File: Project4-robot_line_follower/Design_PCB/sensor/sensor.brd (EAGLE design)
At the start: 134.9 x 70.1 mm, 57 parts

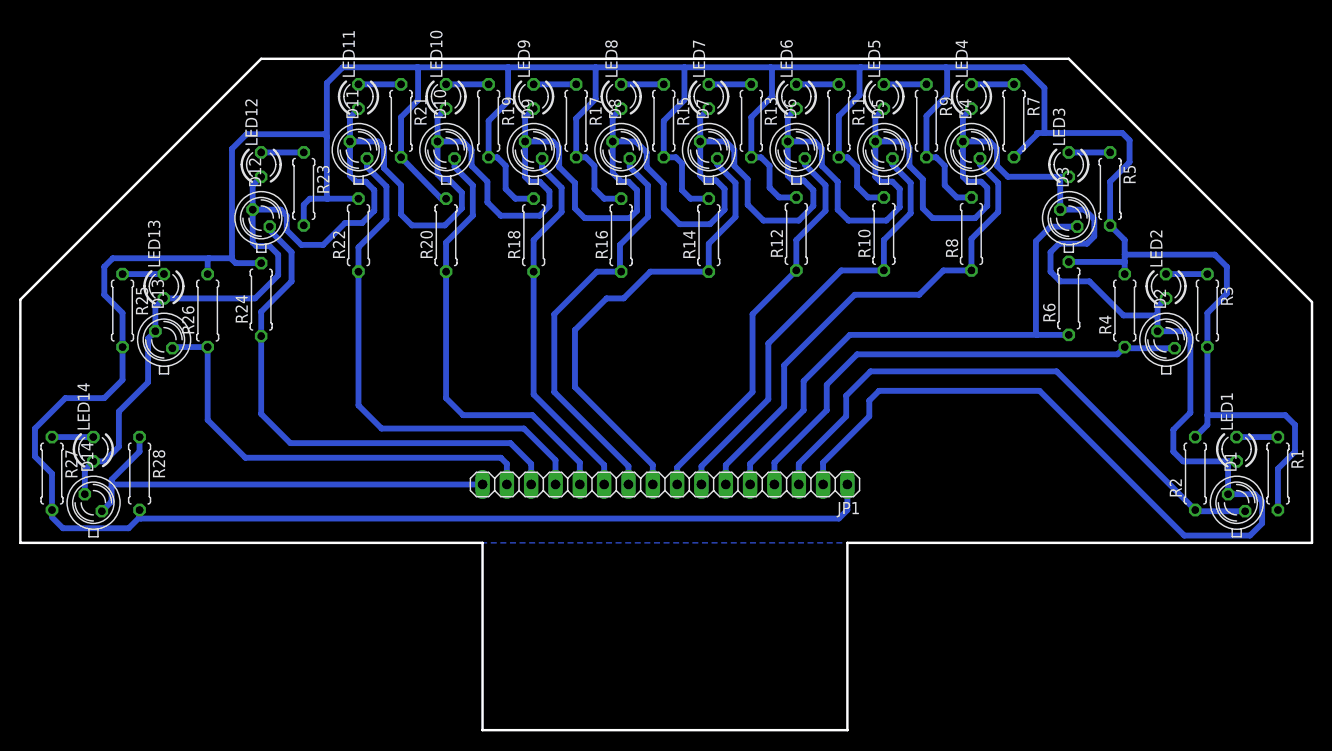
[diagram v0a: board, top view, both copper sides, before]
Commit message: rename file
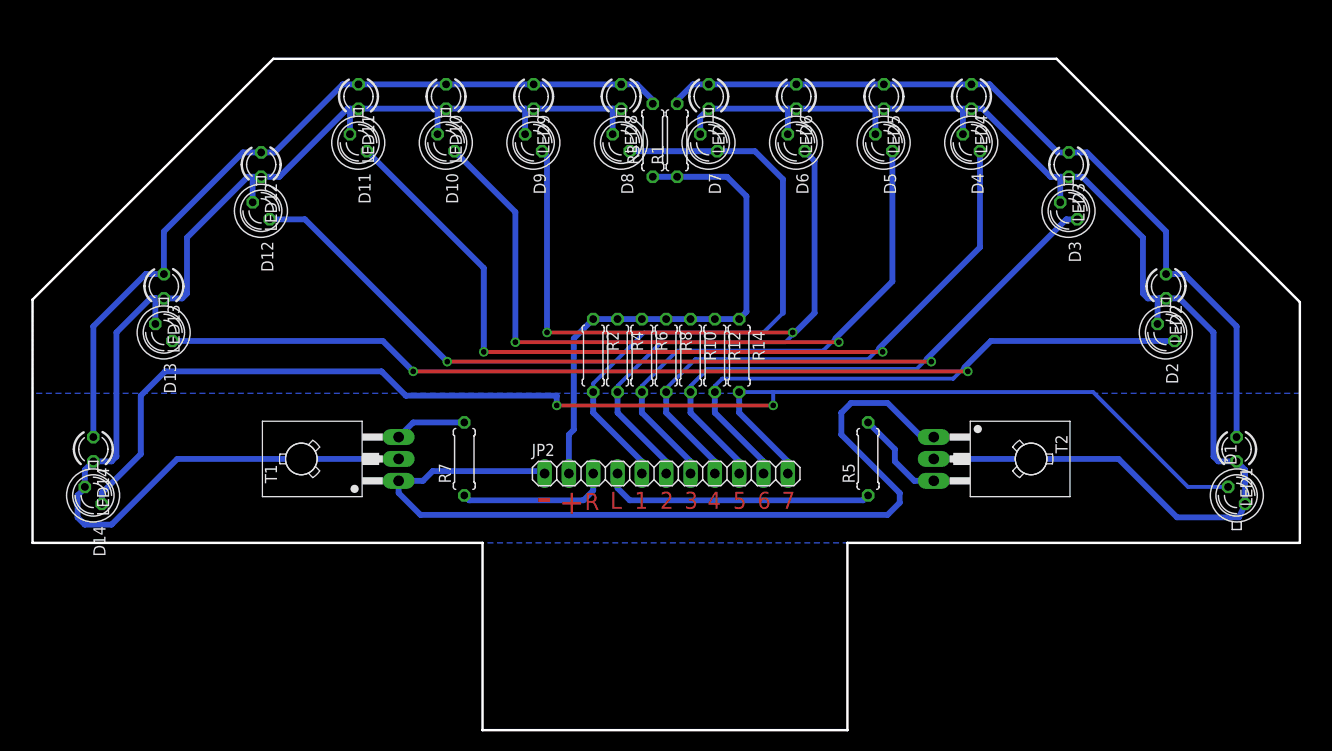
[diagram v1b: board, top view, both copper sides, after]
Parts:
- removed JP1: (no value), pinhead:1X16
- removed R11, R13, R15, R17, R19, R21, R23, R25, R27, R9: 470, rcl:0207/7
- removed R16, R18, R20, R22, R24, R26, R28: 22K, rcl:0207/7
- added JP2: (no value), pinhead:1X11
- added T1, T2: BD139, transistor:TO126
- R1, R3: value 470 -> 56
- R5, R7: value 470 -> 330
- moved R1 71.7 mm to (88.3, 72.1), turned to 90 degrees
- moved R7 67.4 mm to (66.0, 38.9), turned to 90 degrees
- moved R2 64.1 mm to (79.5, 49.7), turned to 270 degrees
- moved R3 60.6 mm to (85.7, 72.1), turned to 90 degrees
- moved R4 53.2 mm to (82.0, 49.7), turned to 270 degrees
- moved R6 45.0 mm to (84.6, 49.7), turned to 270 degrees
- moved R5 37.9 mm to (108.2, 38.9), turned to 90 degrees
- moved R8 34.3 mm to (87.1, 49.7), turned to 270 degrees
- moved R10 23.9 mm to (89.7, 49.7), turned to 270 degrees
- moved R12 15.3 mm to (92.2, 49.7), turned to 270 degrees
- moved R14 13.0 mm to (94.7, 49.7), turned to 270 degrees
- moved D1 0.76 mm to (146.7, 35.1)
- moved D10 0.76 mm to (64.1, 71.9), turned to 270 degrees
- moved D11 0.76 mm to (55.0, 71.9), turned to 270 degrees
- moved D12 0.76 mm to (44.8, 64.8), turned to 270 degrees
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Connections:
- removed net 10: D10.A, JP1.12, R20.1
- removed net 11: D11.A, JP1.13, R22.1
- removed net 12: D12.A, JP1.14, R24.1
- removed net 13: D13.A, JP1.15, R26.1
- removed net 14: D14.A, JP1.16, R28.1
- removed net 8: D8.A, JP1.10, R16.1
- removed net 9: D9.A, JP1.11, R18.1
- removed net N$11: LED6.K, R11.1
- removed net N$13: LED7.K, R13.1
- removed net N$15: LED8.K, R15.1
- removed net N$17: LED9.K, R17.1
- removed net N$19: LED10.K, R19.1
- removed net N$21: LED11.K, R21.1
- removed net N$23: LED12.K, R23.1
- removed net N$25: LED13.K, R25.1
- removed net N$27: LED14.K, R27.1
- removed net N$3: LED2.K, R3.1
- removed net N$5: LED3.K, R5.1
- removed net N$7: LED4.K, R7.1
- removed net N$9: LED5.K, R9.1
- new net D_KA: JP2.4, R5.1
- new net D_KI: JP2.3, R7.1
- new net LED_KA: LED1.A, LED2.A, LED3.A, LED4.A, LED5.A, LED6.A, LED7.A, R1.2
- new net LED_KI: LED10.A, LED11.A, LED12.A, LED13.A, LED14.A, LED8.A, LED9.A, R3.2
- new net N$2: R5.2, T2.3
- new net T_KA: D1.A, D2.A, D3.A, D4.A, D5.A, D6.A, D7.A, LED1.K, LED2.K, LED3.K, LED4.K, LED5.K, LED6.K, LED7.K, T2.2
- new net T_KI: D10.A, D11.A, D12.A, D13.A, D14.A, D8.A, D9.A, LED10.K, LED11.K, LED12.K, LED13.K, LED14.K, LED8.K, LED9.K, T1.2
- net 1: now also D7.K, D8.K, JP2.5, R2.2; no longer D1.A, JP1.3, R2.1
- net 2: now also D6.K, D9.K, JP2.6, R4.2; no longer D2.A, JP1.4, R4.1
- net 3: now also D10.K, D5.K, JP2.7, R6.2; no longer D3.A, JP1.5, R6.1
- net 4: now also D11.K, D4.K, JP2.8, R8.2; no longer D4.A, JP1.6, R8.1
- net 5: now also D12.K, D3.K, JP2.9, R10.2; no longer D5.A, JP1.7, R10.1
- net 5V: now also JP2.2, R1.1, R10.1, R12.1, R14.1, R2.1, R3.1, R4.1, R6.1, R8.1; no longer D1.K, D10.K, D11.K, D12.K, D13.K, D14.K, D2.K, D3.K, D4.K, D5.K, D6.K, D7.K, D8.K, D9.K, JP1.2, LED1.A, LED10.A, LED11.A, LED12.A, LED13.A, LED14.A, LED2.A, LED3.A, LED4.A, LED5.A, LED6.A, LED7.A, LED8.A, LED9.A
- net 6: now also D13.K, D2.K, JP2.10, R12.2; no longer D6.A, JP1.8, R12.1
- net 7: now also D1.K, D14.K, JP2.11, R14.2; no longer D7.A, JP1.9, R14.1
- net GND: now also JP2.1, T1.1, T2.1; no longer JP1.1, R1.2, R10.2, R11.2, R12.2, R13.2, R14.2, R15.2, R16.2, R17.2, R18.2, R19.2, R2.2, R20.2, R21.2, R22.2, R23.2, R24.2, R25.2, R26.2, R27.2, R28.2, R3.2, R4.2, R5.2, R6.2, R7.2, R8.2, R9.2
- net N$1: now also R7.2, T1.3; no longer LED1.K, R1.1
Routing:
- net GND: track 473.1 -> 94.3 mm
- net 5V: track 433.3 -> 56.2 mm
- net T_KI: track 0.00 -> 140.7 mm
- net T_KA: track 0.00 -> 138.8 mm
- net 6: track 41.3 -> 146.1 mm, vias 0 -> 2
- net 7: track 49.7 -> 149.3 mm, vias 0 -> 2
- net 5: track 46.5 -> 134.7 mm, vias 0 -> 2
- net LED_KA: track 0.00 -> 84.1 mm
- net LED_KI: track 0.00 -> 84.1 mm
- net 4: track 52.3 -> 128.1 mm, vias 0 -> 2
- net 3: track 57.6 -> 112.4 mm, vias 0 -> 2
- net 12: track 54.3 -> 0.00 mm
- net 11: track 53.3 -> 0.00 mm
- net 14: track 48.2 -> 0.00 mm
- net 13: track 46.7 -> 0.00 mm
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- added copper zone on layer 16, net 5V
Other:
- board size 134.9 x 70.1 mm -> 132.3 x 70.1 mm
- board text added: "+"
- board text added: "-"
- board text added: "1"
- board text added: "2"
- board text added: "3"
- board text added: "4"
- board text added: "5"
- board text added: "6"
- board text added: "7"
- board text added: "L"
- board text added: "R"
